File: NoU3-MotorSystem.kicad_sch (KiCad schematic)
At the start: 38 parts, among them J1 JST SR/SZ, J10 JST SR/SZ, J13 JST SR/SZ, J15 Barrel_Jack, J16 VIN, J17 JST SR/SZ, J18 GND, J4 JST SR/SZ, J7 JST SR/SZ, Q1 AO3401A, U10 PCA9685BS, U15 SY8113BADC, U16 SY8113BADC, U8 5.8 ZSPT

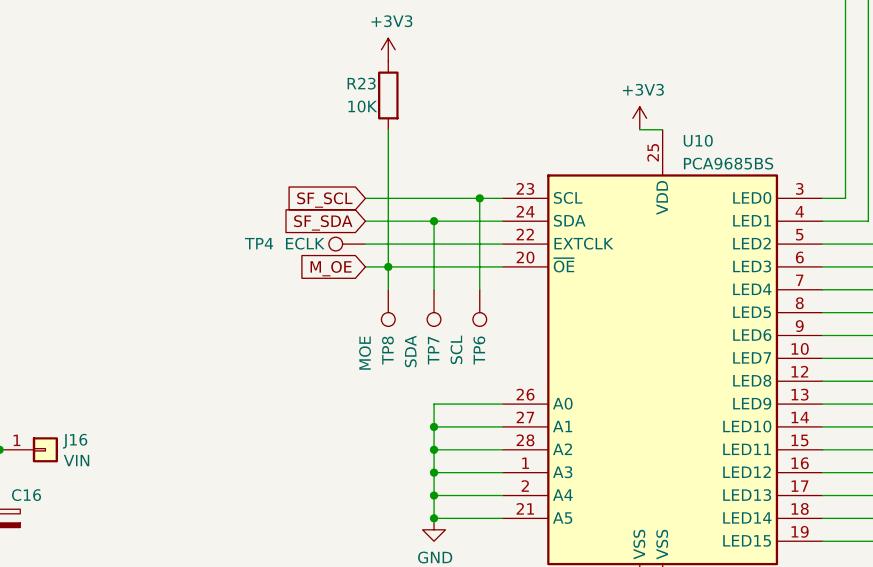
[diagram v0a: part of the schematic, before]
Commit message: bumped version to NoU3.5
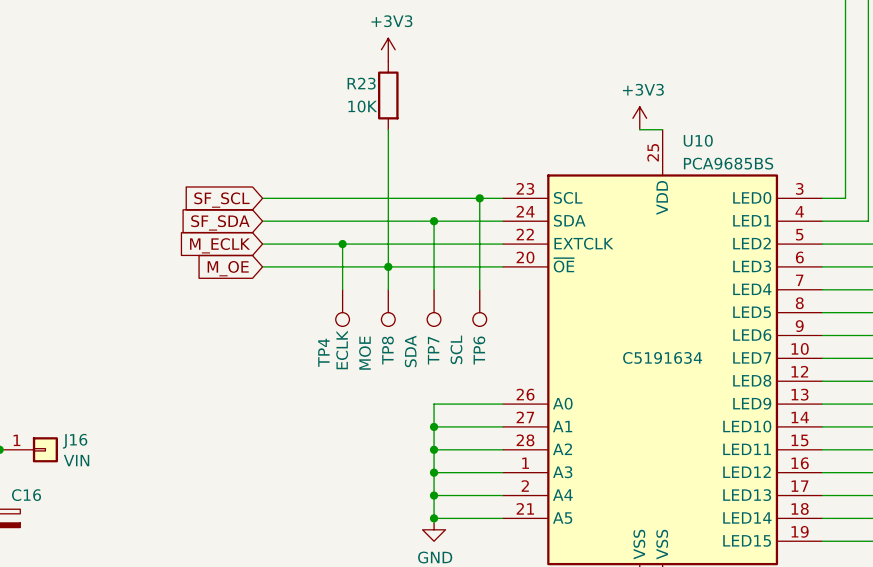
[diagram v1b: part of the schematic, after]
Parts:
- U10: LCSC (none) -> C5191634
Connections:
- net M_ECLK: now reaches TP4.1, U10.22 (EXTCLK)
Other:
- moved on the sheet: TP4
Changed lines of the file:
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@@
 	)
 	(junction
+		(at 110.49 86.36)
+		(diameter 0)
+		(color 0 0 0 0)
+	)
+	(junction
 		(at 30.48 168.91)
 		(diameter 0)
@@
 	(wire
 		(pts
-			(xy 113.03 88.9) (xy 115.57 88.9)
+			(xy 101.6 88.9) (xy 115.57 88.9)
 		)
 		(stroke
@@
 	(wire
 		(pts
+			(xy 110.49 91.44) (xy 110.49 86.36)
+		)
+		(stroke
+			(width 0)
+			(type default)
+		)
+	)
+	(wire
+		(pts
 			(xy 168.91 83.82) (xy 163.83 83.82)
 		)
@@
 	(wire
 		(pts
+			(xy 110.49 86.36) (xy 128.27 86.36)
+		)
+		(stroke
+			(width 0)
+			(type default)
+		)
+	)
+	(wire
+		(pts
 			(xy 215.9 92.71) (xy 232.41 92.71)
 		)
@@
 	(wire
 		(pts
-			(xy 113.03 81.28) (xy 125.73 81.28)
+			(xy 101.6 81.28) (xy 125.73 81.28)
 		)
 		(stroke
@@
 	(wire
 		(pts
+			(xy 101.6 86.36) (xy 110.49 86.36)
+		)
+		(stroke
+			(width 0)
+			(type default)
+		)
+	)
+	(wire
+		(pts
 			(xy 143.51 73.66) (xy 146.05 73.66)
 		)
@@
 	(wire
 		(pts
-			(xy 113.03 83.82) (xy 120.65 83.82)
+			(xy 101.6 83.82) (xy 120.65 83.82)
 		)
 		(stroke
@@
 	(wire
 		(pts
-			(xy 113.03 86.36) (xy 128.27 86.36)
-		)
-		(stroke
-			(width 0)
-			(type default)
-		)
-	)
-	(wire
-		(pts
 			(xy 48.26 171.45) (xy 59.69 171.45)
 		)
@@
 	(global_label "SF_SDA"
 		(shape input)
-		(at 113.03 83.82 180)
+		(at 101.6 83.82 180)
 		(fields_autoplaced yes)
 		(effects
@@
 		)
 		(property "Intersheetrefs" "${INTERSHEET_REFS}"
-			(at 103.9446 83.82 0)
+			(at 92.5146 83.82 0)
 			(effects
 				(font
@@
 	(global_label "SF_SCL"
 		(shape input)
-		(at 113.03 81.28 180)
+		(at 101.6 81.28 180)
 		(fields_autoplaced yes)
 		(effects
@@
 		)
 		(property "Intersheetrefs" "${INTERSHEET_REFS}"
-			(at 104.0051 81.28 0)
+			(at 92.5751 81.28 0)
 			(effects
 				(font
@@
 		)
 	)
+	(global_label "M_ECLK"
+		(shape input)
+		(at 101.6 86.36 180)
+		(fields_autoplaced yes)
+		(effects
+			(font
+				(size 1.27 1.27)
+			)
+			(justify right)
+		)
+		(property "Intersheetrefs" "${INTERSHEET_REFS}"
+			(at 92.1329 86.36 0)
+			(effects
+				(font
+					(size 1.27 1.27)
+				)
+				(justify right)
+				(hide yes)
+			)
+		)
+	)
 	(global_label "M_OE"
 		(shape input)
-		(at 113.03 88.9 180)
+		(at 101.6 88.9 180)
 		(fields_autoplaced yes)
 		(effects
@@
 		)
 		(property "Intersheetrefs" "${INTERSHEET_REFS}"
-			(at 105.8005 88.9 0)
+			(at 94.3705 88.9 0)
 			(effects
 				(font
@@
 	(symbol
 		(lib_id "Connector:TestPoint")
-		(at 113.03 86.36 90)
+		(at 110.49 91.44 180)
 		(unit 1)
 		(exclude_from_sim no)
@@
 		(dnp no)
 		(property "Reference" "TP4"
-			(at 102.87 86.36 90)
+			(at 108.458 96.774 90)
 			(effects
 				(font
@@
 		)
 		(property "Value" "ECLK"
-			(at 108.458 86.36 90)
+			(at 110.49 96.012 90)
 			(effects
 				(font
@@
 		)
 		(property "Footprint" "AlfredoFootprints:PogoPad1"
-			(at 113.03 81.28 0)
+			(at 105.41 91.44 0)
 			(effects
 				(font
@@
 		)
 		(property "Datasheet" "~"
-			(at 113.03 81.28 0)
+			(at 105.41 91.44 0)
 			(effects
 				(font
@@
 		)
 		(property "Description" ""
-			(at 113.03 86.36 0)
+			(at 110.49 91.44 0)
 			(effects
 				(font
@@
 		)
 		(property "LCSC" "~"
-			(at 113.03 86.36 0)
+			(at 110.49 91.44 0)
 			(effects
 				(font
@@
 			)
 		)
+		(property "LCSC" " C5191634"
+			(at 146.05 99.06 0)
+			(effects
+				(font
+					(size 1.27 1.27)
+				)
+			)
+		)
